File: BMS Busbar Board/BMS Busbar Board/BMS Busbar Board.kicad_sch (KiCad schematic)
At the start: 17 parts, among them J1 Conn_01x05_MountingPin, J2 Conn_01x05_MountingPin

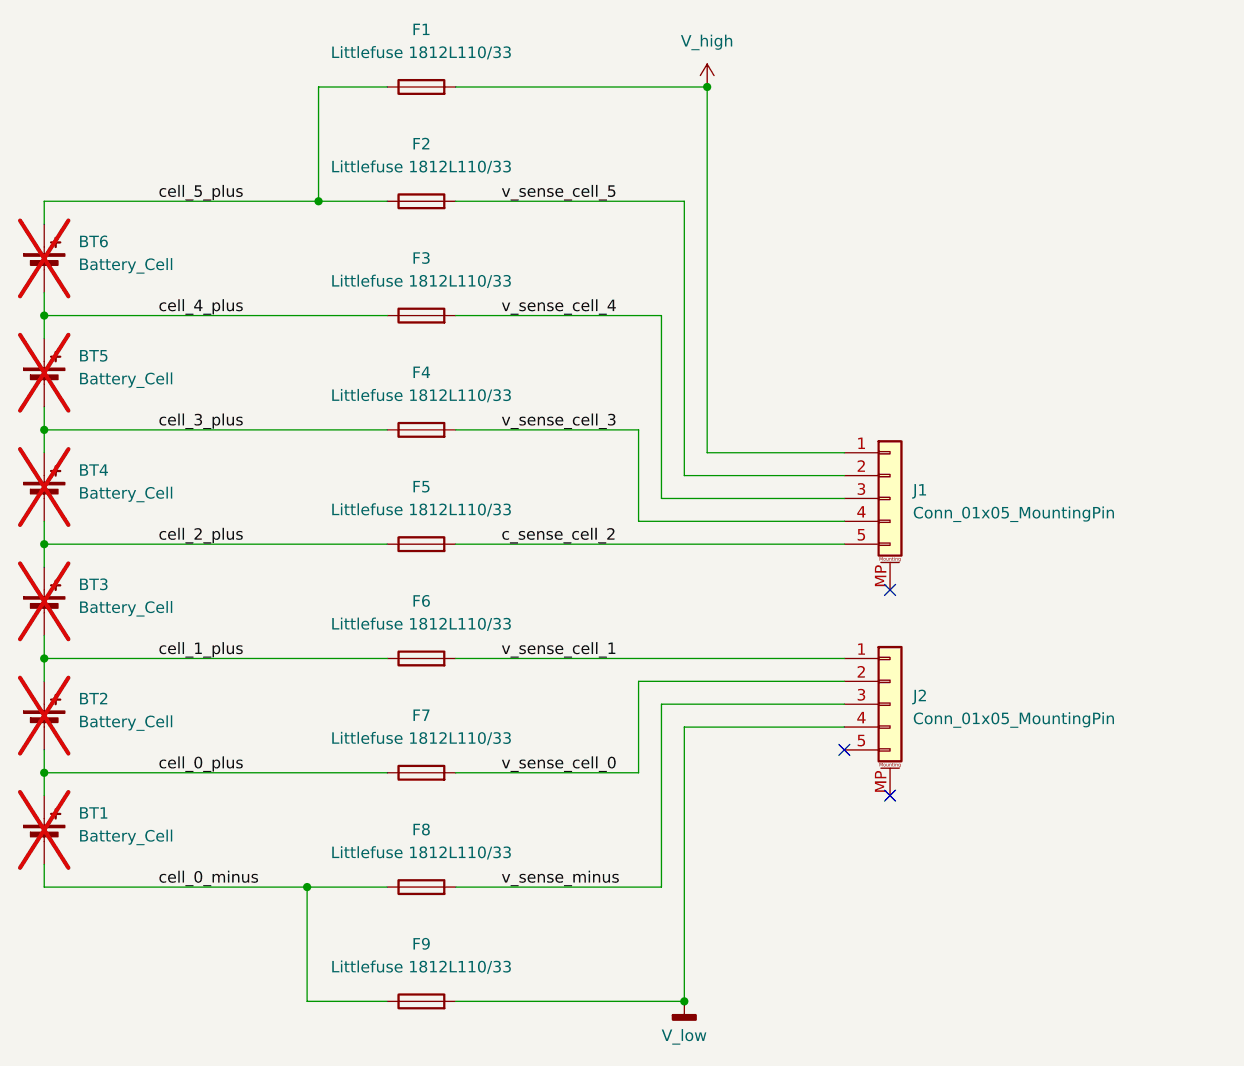
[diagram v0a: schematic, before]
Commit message: busbar pcb complete (with violations)
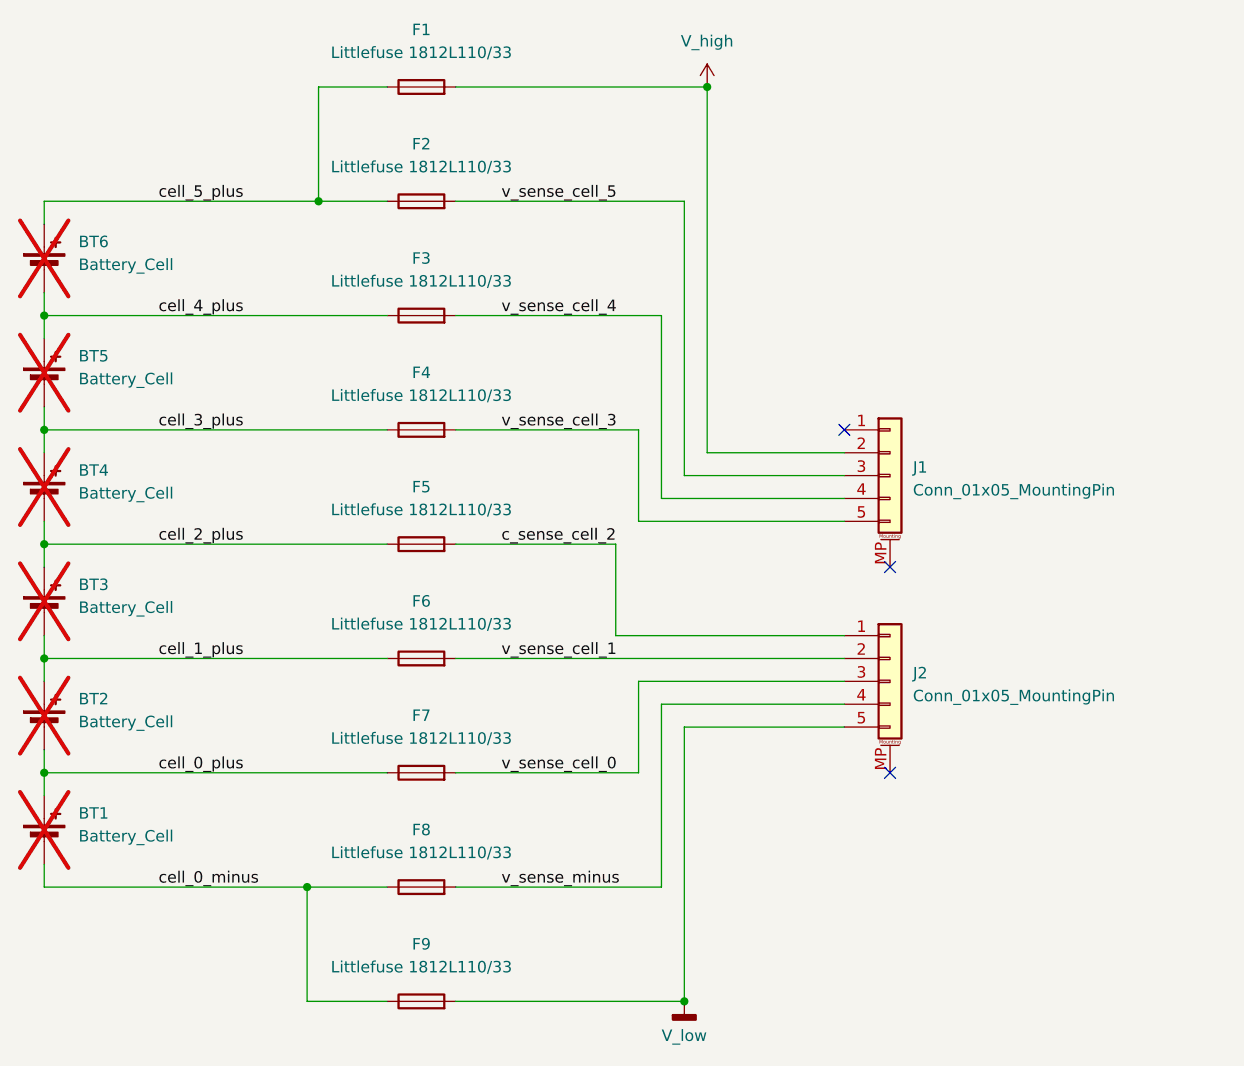
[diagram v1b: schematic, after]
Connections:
- net V_high: now also J1.2 (Pin_2); no longer J1.1 (Pin_1)
- net V_low: now also J2.5 (Pin_5); no longer J2.4 (Pin_4)
- net c_sense_cell_2: now also J2.1 (Pin_1); no longer J1.5 (Pin_5)
- net v_sense_cell_0: now also J2.3 (Pin_3); no longer J2.2 (Pin_2)
- net v_sense_cell_1: now also J2.2 (Pin_2); no longer J2.1 (Pin_1)
- net v_sense_cell_3: now also J1.5 (Pin_5); no longer J1.4 (Pin_4)
- net v_sense_cell_4: now also J1.4 (Pin_4); no longer J1.3 (Pin_3)
- net v_sense_cell_5: now also J1.3 (Pin_3); no longer J1.2 (Pin_2)
- net v_sense_minus: now also J2.4 (Pin_4); no longer J2.3 (Pin_3)
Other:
- moved on the sheet: J1, J2
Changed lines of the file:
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@@
 	)
 	(no_connect
-		(at 157.48 106.68)
+		(at 157.48 104.14)
 	)
 	(no_connect
-		(at 157.48 83.82)
+		(at 157.48 81.28)
 	)
 	(no_connect
-		(at 152.4 101.6)
+		(at 152.4 66.04)
+	)
+	(wire
+		(pts
+			(xy 137.16 68.58) (xy 152.4 68.58)
+		)
+		(stroke
+			(width 0)
+			(type default)
+		)
 	)
 	(wire
@@
 	(wire
 		(pts
-			(xy 152.4 93.98) (xy 129.54 93.98)
+			(xy 134.62 99.06) (xy 152.4 99.06)
 		)
 		(stroke
@@
 	(wire
 		(pts
-			(xy 137.16 68.58) (xy 152.4 68.58)
+			(xy 129.54 93.98) (xy 152.4 93.98)
 		)
 		(stroke
@@
 	(wire
 		(pts
+			(xy 152.4 88.9) (xy 127 88.9)
+		)
+		(stroke
+			(width 0)
+			(type default)
+		)
+	)
+	(wire
+		(pts
+			(xy 109.22 91.44) (xy 152.4 91.44)
+		)
+		(stroke
+			(width 0)
+			(type default)
+		)
+	)
+	(wire
+		(pts
 			(xy 63.5 40.64) (xy 63.5 43.18)
 		)
@@
 	(wire
 		(pts
-			(xy 109.22 78.74) (xy 152.4 78.74)
-		)
-		(stroke
-			(width 0)
-			(type default)
-		)
-	)
-	(wire
-		(pts
 			(xy 93.98 27.94) (xy 93.98 40.64)
 		)
@@
 	(wire
 		(pts
+			(xy 127 88.9) (xy 127 78.74)
+		)
+		(stroke
+			(width 0)
+			(type default)
+		)
+	)
+	(wire
+		(pts
 			(xy 63.5 114.3) (xy 63.5 116.84)
 		)
@@
 	(wire
 		(pts
-			(xy 152.4 99.06) (xy 134.62 99.06)
-		)
-		(stroke
-			(width 0)
-			(type default)
-		)
-	)
-	(wire
-		(pts
 			(xy 134.62 40.64) (xy 109.22 40.64)
 		)
@@
 	(wire
 		(pts
-			(xy 152.4 76.2) (xy 129.54 76.2)
-		)
-		(stroke
-			(width 0)
-			(type default)
-		)
-	)
-	(wire
-		(pts
 			(xy 101.6 129.54) (xy 92.71 129.54)
 		)
@@
 	(wire
 		(pts
-			(xy 152.4 96.52) (xy 132.08 96.52)
-		)
-		(stroke
-			(width 0)
-			(type default)
-		)
-	)
-	(wire
-		(pts
 			(xy 63.5 63.5) (xy 63.5 66.04)
 		)
@@
 	(wire
 		(pts
+			(xy 109.22 78.74) (xy 127 78.74)
+		)
+		(stroke
+			(width 0)
+			(type default)
+		)
+	)
+	(wire
+		(pts
 			(xy 101.6 53.34) (xy 63.5 53.34)
 		)
@@
 	(wire
 		(pts
-			(xy 109.22 91.44) (xy 152.4 91.44)
+			(xy 129.54 76.2) (xy 152.4 76.2)
 		)
 		(stroke
@@
 	(wire
 		(pts
+			(xy 132.08 96.52) (xy 152.4 96.52)
+		)
+		(stroke
+			(width 0)
+			(type default)
+		)
+	)
+	(wire
+		(pts
+			(xy 132.08 73.66) (xy 152.4 73.66)
+		)
+		(stroke
+			(width 0)
+			(type default)
+		)
+	)
+	(wire
+		(pts
 			(xy 137.16 27.94) (xy 137.16 68.58)
 		)
@@
 	(wire
 		(pts
+			(xy 134.62 71.12) (xy 152.4 71.12)
+		)
+		(stroke
+			(width 0)
+			(type default)
+		)
+	)
+	(wire
+		(pts
 			(xy 109.22 104.14) (xy 129.54 104.14)
 		)
@@
 	(wire
 		(pts
-			(xy 132.08 73.66) (xy 152.4 73.66)
-		)
-		(stroke
-			(width 0)
-			(type default)
-		)
-	)
-	(wire
-		(pts
 			(xy 109.22 53.34) (xy 132.08 53.34)
-		)
-		(stroke
-			(width 0)
-			(type default)
-		)
-	)
-	(wire
-		(pts
-			(xy 152.4 71.12) (xy 134.62 71.12)
 		)
 		(stroke
@@
 	(symbol
 		(lib_id "Connector_Generic_MountingPin:Conn_01x05_MountingPin")
-		(at 157.48 96.52 0)
+		(at 157.48 93.98 0)
 		(unit 1)
 		(exclude_from_sim no)
@@
 		(dnp no)
 		(property "Reference" "J2"
+			(at 160.02 93.0655 0)
+			(effects
+				(font
+					(size 1.27 1.27)
+				)
+				(justify left)
+			)
+		)
+		(property "Value" "Conn_01x05_MountingPin"
 			(at 160.02 95.6055 0)
 			(effects
@@
 			)
 		)
-		(property "Value" "Conn_01x05_MountingPin"
-			(at 160.02 98.1455 0)
-			(effects
-				(font
-					(size 1.27 1.27)
-				)
-				(justify left)
-			)
-		)
 		(property "Footprint" "FS_4_Global_Footprint_Library:CON_5019510550"
-			(at 157.48 96.52 0)
+			(at 157.48 93.98 0)
 			(effects
 				(font
@@
 		)
 		(property "Datasheet" "~"
-			(at 157.48 96.52 0)
+			(at 157.48 93.98 0)
 			(effects
 				(font
@@
 		)
 		(property "Description" "Generic connectable mounting pin connector, single row, 01x05, script generated (kicad-library-utils/schlib/autogen/connector/)"
-			(at 157.48 96.52 0)
+			(at 157.48 93.98 0)
 			(effects
 				(font
@@
 	(symbol
 		(lib_id "Connector_Generic_MountingPin:Conn_01x05_MountingPin")
-		(at 157.48 73.66 0)
+		(at 157.48 71.12 0)
 		(unit 1)
 		(exclude_from_sim no)
@@
 		(dnp no)
 		(property "Reference" "J1"
+			(at 160.02 70.2055 0)
+			(effects
+				(font
+					(size 1.27 1.27)
+				)
+				(justify left)
+			)
+		)
+		(property "Value" "Conn_01x05_MountingPin"
 			(at 160.02 72.7455 0)
 			(effects
@@
 			)
 		)
-		(property "Value" "Conn_01x05_MountingPin"
-			(at 160.02 75.2855 0)
-			(effects
-				(font
-					(size 1.27 1.27)
-				)
-				(justify left)
-			)
-		)
 		(property "Footprint" "FS_4_Global_Footprint_Library:CON_5019510550"
-			(at 157.48 73.66 0)
+			(at 157.48 71.12 0)
 			(effects
 				(font
@@
 		)
 		(property "Datasheet" "~"
-			(at 157.48 73.66 0)
+			(at 157.48 71.12 0)
 			(effects
 				(font
@@
 		)
 		(property "Description" "Generic connectable mounting pin connector, single row, 01x05, script generated (kicad-library-utils/schlib/autogen/connector/)"
-			(at 157.48 73.66 0)
-			(effects
-				(font
+			(at 157.48 71.12 0)
+			(effects
+				(font

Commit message: imported and placed new connector
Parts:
- J1, J2: footprint FS_4_Global_Footprint_Library:CON_5019510550 -> FS_4_Global_Footprint_Library:512810598
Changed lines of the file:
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@@
 			)
 		)
-		(property "Footprint" "FS_4_Global_Footprint_Library:CON_5019510550"
+		(property "Footprint" "FS_4_Global_Footprint_Library:512810598"
 			(at 157.48 93.98 0)
 			(effects
@@
 			)
 		)
-		(property "Footprint" "FS_4_Global_Footprint_Library:CON_5019510550"
+		(property "Footprint" "FS_4_Global_Footprint_Library:512810598"
 			(at 157.48 71.12 0)
 			(effects
